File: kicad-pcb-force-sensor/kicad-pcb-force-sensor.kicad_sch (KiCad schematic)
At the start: 20 parts, among them J1 Power, J2 Digital/PWM, J3 Analog, J4 Digital/PWM, M1 Motor_Servo, U3 KY-040

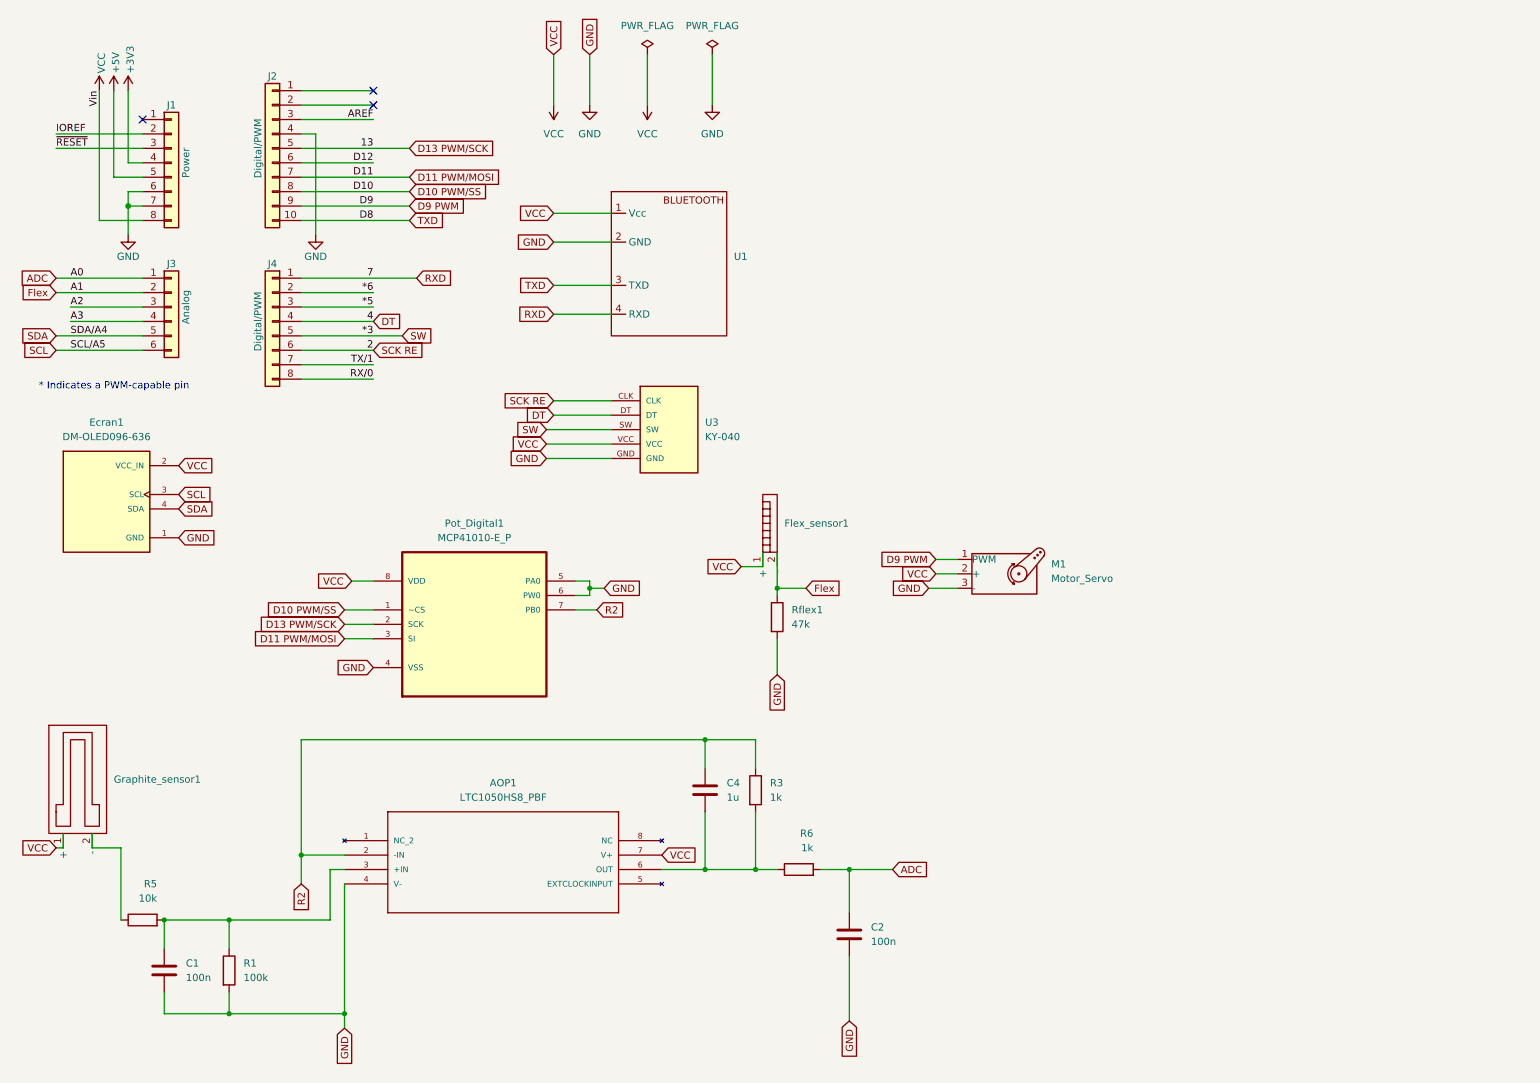
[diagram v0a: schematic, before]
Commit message: partie Kicad
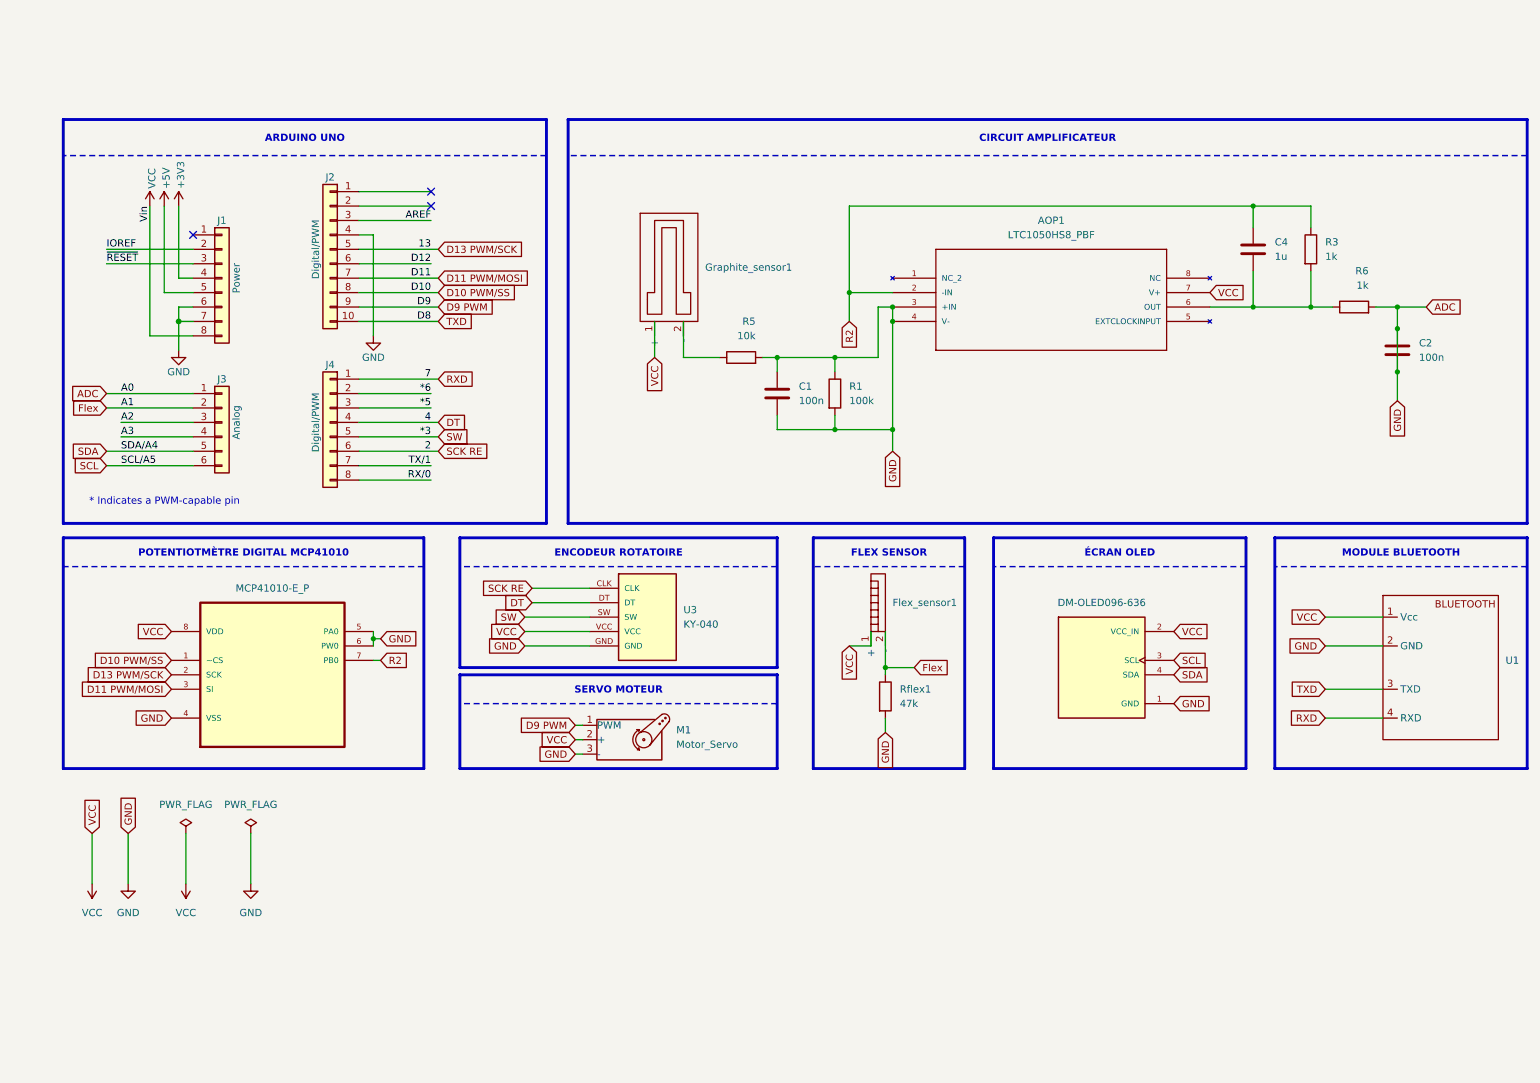
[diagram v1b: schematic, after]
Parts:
- renumbered Ecran1 to DM-OLED096-636
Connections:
- net ADC is gone; now on net GND: C2.2, J3.1 (Pin_1), R6.2
- net GND: now also AOP1.3 (+IN), C1.2, R1.1, R5.2
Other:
- moved on the sheet: AOP1, C1, C2, C4, DM-OLED096-636, Flex_sensor1, Graphite_sensor1, J1, J2, J3, J4, M1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
